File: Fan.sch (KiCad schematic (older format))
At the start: 0 parts

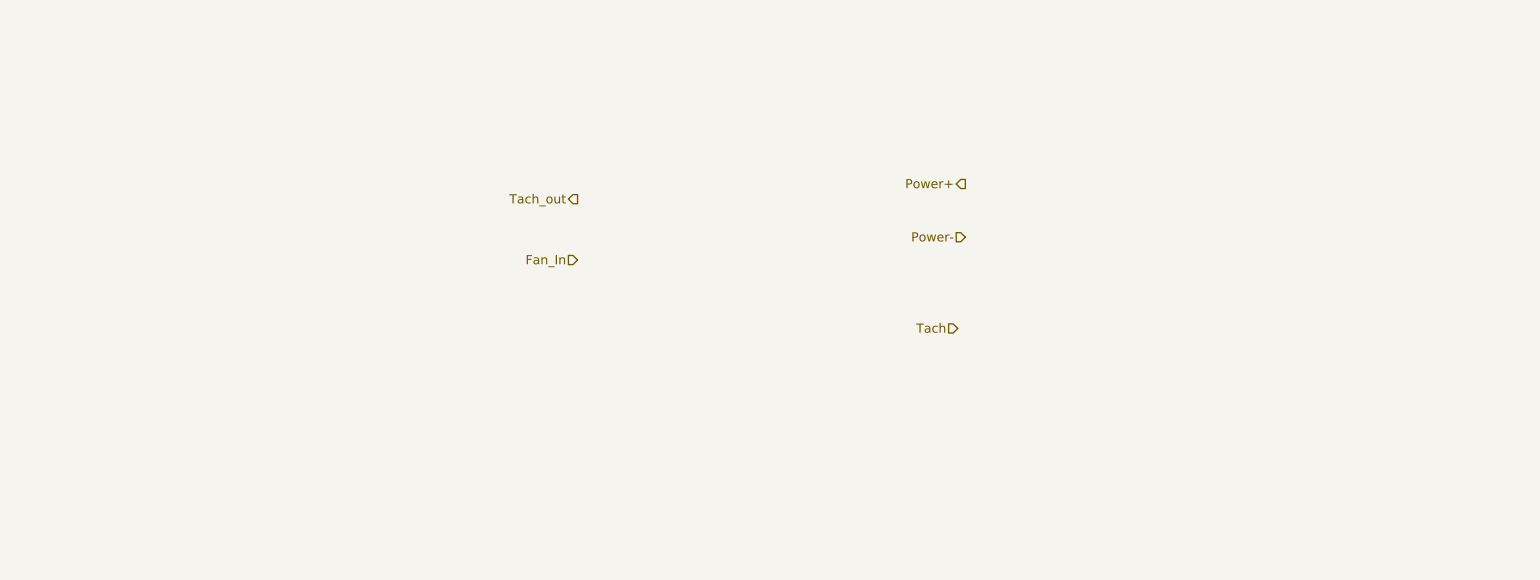
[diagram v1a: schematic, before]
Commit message: Fan Module details
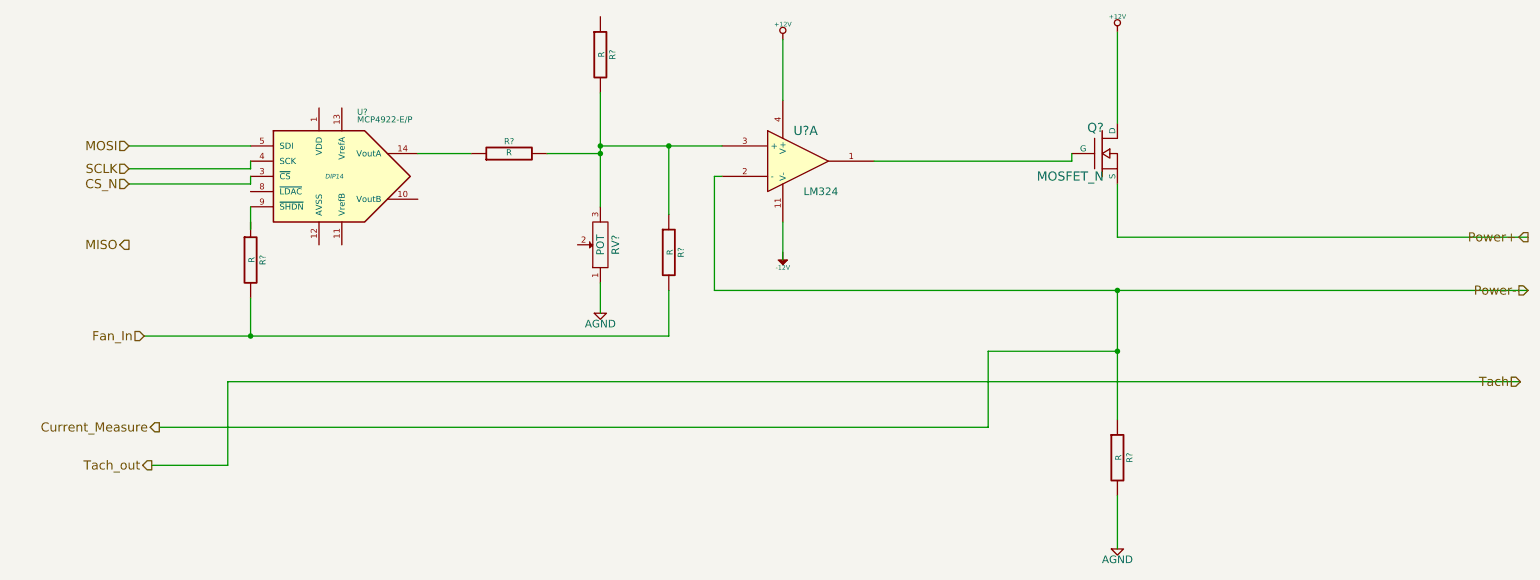
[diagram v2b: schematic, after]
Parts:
- added Q?: MOSFET_N, ~, symbol MOSFET_N
- added R? (x5): R, ~, symbol R
- added RV?: POT, ~, symbol POT
- added U?: LM324, symbol LM324
- added U?: MCP4922-E/P, DIP14, symbol MCP4922-E/P
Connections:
- net labels added: +12V, -12V, AGND, CS_N, Current_Measure, MISO, MOSI, SCLK
- wire segments 0 -> 33
